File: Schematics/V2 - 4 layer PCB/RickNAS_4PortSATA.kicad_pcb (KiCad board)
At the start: 4 copper layers, 136 x 93 mm, 37 parts, among them J1 2227595-1, J10 10076579-002C-TRLF, J2 Conn_01x03, J3 Conn_01x03, J6 POWER, J7 10076579-002C-TRLF, J8 10076579-002C-TRLF, J9 10076579-002C-TRLF, U1 CH32V003FxPx, U2 TLV1117-33

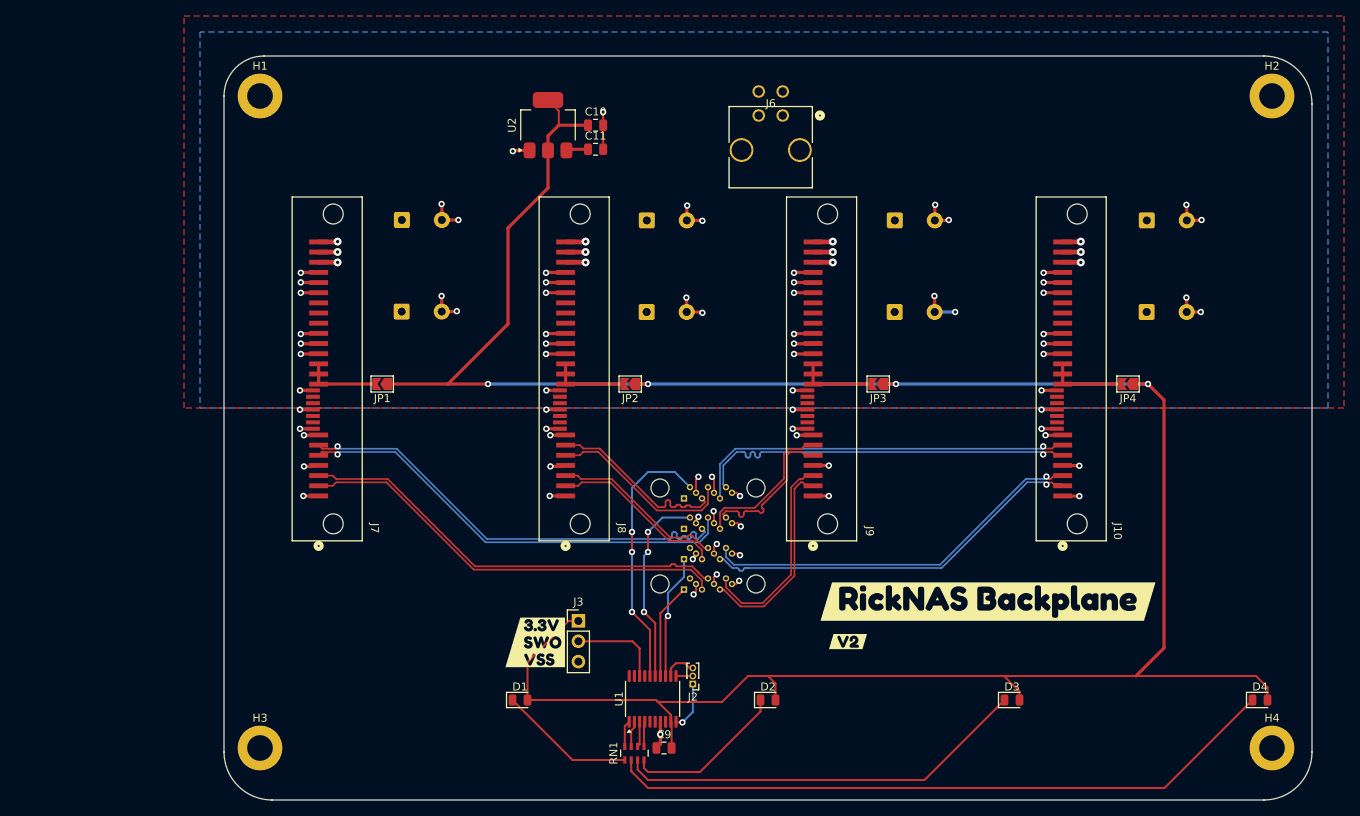
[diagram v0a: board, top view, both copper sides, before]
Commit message: ran erc
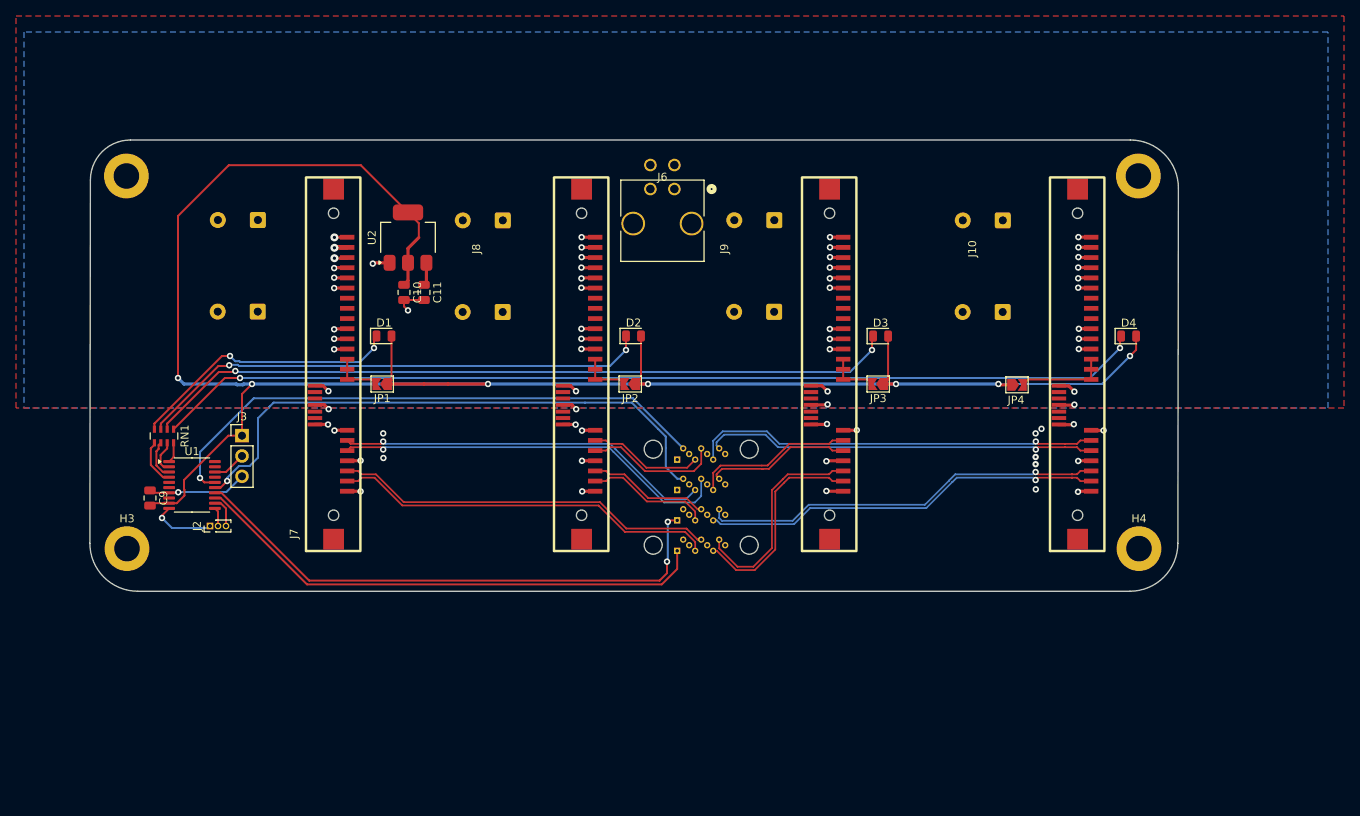
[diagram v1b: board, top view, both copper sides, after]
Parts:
- removed kibuzzard-6986109D: G***, kibuzzard-6986109D
- added kibuzzard-69F8CF71: G***, kibuzzard-69F8CF71, B.Cu at (198.1, 79.0)
- J10, J7, J8, J9: footprint UE_Connector:CONN_10076579-002C-TRLF_AMP -> UE_Connector:91908-291512_SAS_Conn
- kibuzzard-69861090, kibuzzard-698626E9: moved to B.Cu
- moved C9 71.4 mm to (98.8, 83.2), turned to -90 degrees
- moved RN1 70.9 mm to (100.5, 75.5), turned to -90 degrees
- moved J2 63.5 mm to (106.2, 86.8), turned to 90 degrees
- moved U1 63.5 mm to (104.0, 81.6), turned to 0 degrees
- moved D1 48.6 mm to (128.0, 63.0)
- moved D2 48.5 mm to (159.2, 63.0)
- moved D3 48.4 mm to (190.1, 63.0)
- moved D4 48.4 mm to (221.1, 63.0)
- moved J3 48.0 mm to (110.2, 75.5)
- moved kibuzzard-698626E9 39.1 mm to (115.5, 78.0), turned to 180 degrees
- moved C10 31.8 mm to (130.5, 57.5), turned to -90 degrees
- moved H3 30.0 mm to (95.9, 89.6)
- moved H4 30.0 mm to (222.4, 89.6)
- moved C11 27.9 mm to (133.0, 57.5), turned to -90 degrees
- moved U2 22.4 mm to (131.0, 50.7)
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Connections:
- RN1 pad 1: Net-(D1-K) -> Net-(D4-K)
- RN1 pad 2: Net-(D4-K) -> Net-(D3-K)
- RN1 pad 3: Net-(D3-K) -> Net-(D2-K)
- RN1 pad 4: Net-(D2-K) -> Net-(D1-K)
- U1 pad 13: SDataOut -> SDataIn
- U1 pad 14: SDataIn -> SDataOut
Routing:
- net +3.3V: track 307.3 -> 247.2 mm, vias 4 -> 7
- net SDataOut: track 15.6 -> 69.2 mm, vias 1 -> 2
- net SDataIn: track 12.0 -> 65.3 mm
- net SLoad: track 24.8 -> 72.2 mm, vias 3 -> 1
- net Net-(D2-K): track 20.3 -> 64.5 mm, vias 0 -> 2
- net VSS: track 151.8 -> 108.0 mm, vias 79 -> 58
- net Net-(D3-K): track 51.7 -> 94.5 mm, vias 0 -> 2
- net Net-(D4-K): track 84.5 -> 124.0 mm, vias 0 -> 2
- net SClock: track 33.3 -> 71.1 mm, vias 3 -> 1
- net Net-(D1-K): track 17.1 -> 34.3 mm, vias 0 -> 2
- net /RX0+: track 57.3 -> 47.4 mm
- net /RX1+: track 23.4 -> 14.3 mm
- net +12V: track 28.6 -> 20.3 mm
- net SWO: track 11.5 -> 4.22 mm
- net /TX1-: track 21.8 -> 15.2 mm
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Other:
- board size 136 x 93 mm -> 136.1 x 56.4 mm
